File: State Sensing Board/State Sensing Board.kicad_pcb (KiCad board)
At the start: 2 copper layers, 37.1 x 9 mm, 14 parts, among them J1 HallSensor_Conn, U1 AH1815-P, U2 AH1815-P

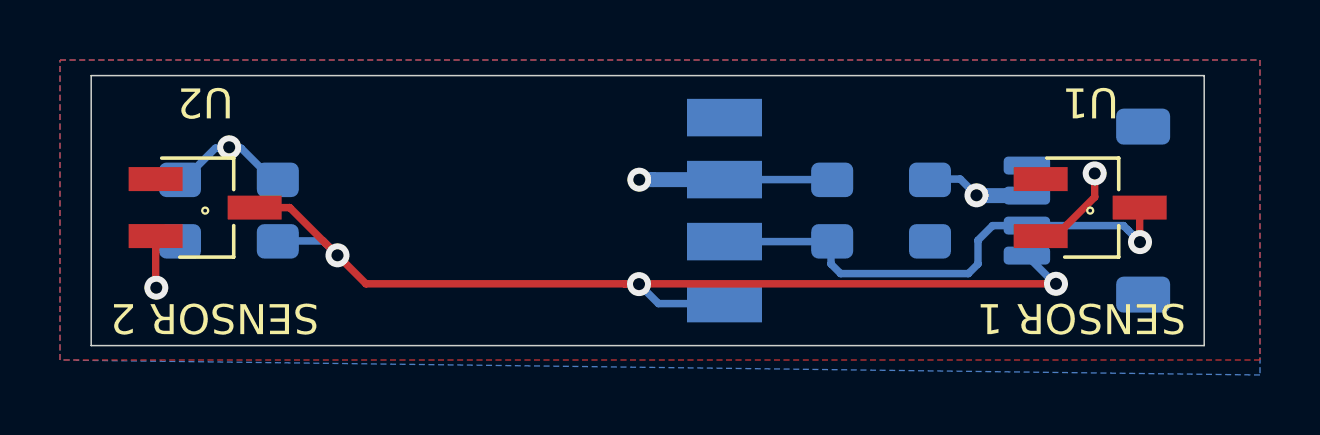
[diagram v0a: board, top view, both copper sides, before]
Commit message: Resize to correct for scale
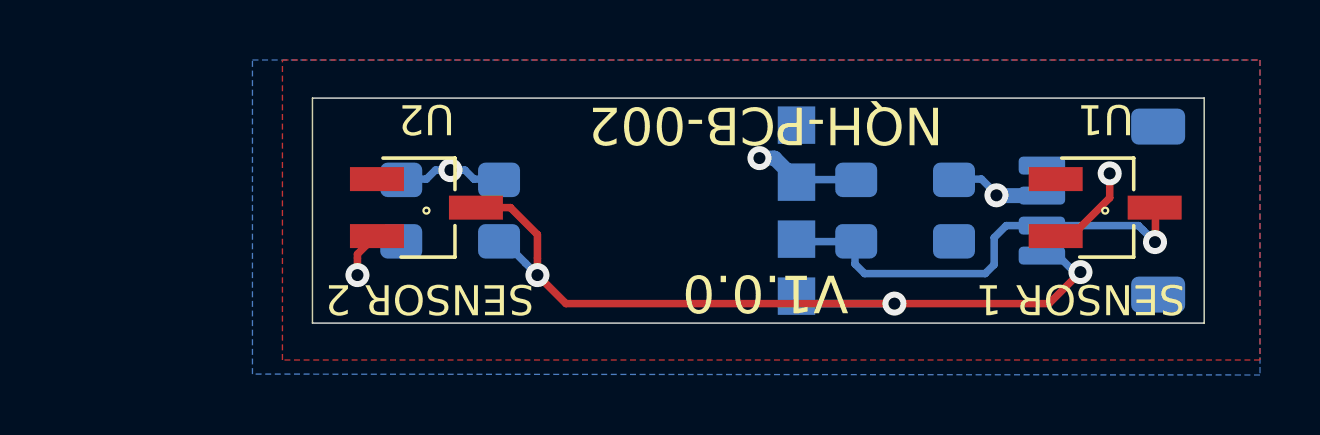
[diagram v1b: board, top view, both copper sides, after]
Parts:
- removed LG1: OSHW Logo, Naquadah_Generator:OSHW_3mm_No_Text
- H1: footprint Naquadah_Generator:MountingSlot_2.7mm_2.7mm_M2.5 -> Naquadah_Generator:MountingSlot_2.2mm_2.2mm_M2.0
- TP101, TP102, TP103, TP104: footprint Frequently Used:Pad_1.25-2.5 -> Naquadah_Generator:Pad_1.25-1.25
- moved C2 7.38 mm to (110.3, 104.5)
- moved R2 7.38 mm to (113.6, 104.5)
- moved U2 7.38 mm to (111.2, 104.4)
- moved H1 5.04 mm to (118.8, 104.5)
- moved TP101 2.41 mm to (123.5, 101.7)
- moved TP104 2.41 mm to (123.5, 107.3)
- moved TP102 2.40 mm to (123.5, 103.5)
- moved TP103 2.40 mm to (123.5, 105.5)
- moved C1 0.80 mm to (128.8, 104.5)
- moved R1 0.80 mm to (125.5, 104.5)
- moved J1 0.50 mm to (133.7, 104.5)
- moved U1 0.50 mm to (133.8, 104.4)
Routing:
- net SENS2: track 34.4 -> 29.3 mm
- net +5V: track 13.5 -> 10.0 mm
- net SENS1: track 17.3 -> 15.2 mm
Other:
- board size 37.1 x 9 mm -> 29.7 x 7.5 mm
